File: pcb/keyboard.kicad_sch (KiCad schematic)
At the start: 130 parts, among them J1 Conn_01x04_Pin, J2 AudioJack4, J3 USB_C_Receptacle_USB2.0_16P, J4 AudioJack4, J5 USB_C_Receptacle_USB2.0_16P, J6 Conn_01x04_Pin, SW1 SW_Push, SW10 SW_Push_45deg, SW11 SW_Push_45deg, SW12 SW_Push_45deg, SW13 SW_Push_45deg, SW14 SW_Push_45deg, SW15 SW_Push_45deg, SW16 SW_Push_45deg, SW17 SW_Push_45deg, SW18 SW_Push_45deg, SW19 SW_Push_45deg, SW2 RotaryEncoder_Switch, SW20 SW_Push_45deg, SW21 SW_Push_45deg, SW22 SW_Push_45deg, SW23 SW_Push_45deg, SW24 SW_Push_45deg, SW26 SW_Push_45deg, SW27 SW_Push_45deg, SW28 SW_Push_45deg, SW29 SW_Push_45deg, SW3 SW_Push_45deg, SW30 SW_Push_45deg, SW31 SW_Push_45deg, SW32 SW_Push_45deg, SW33 SW_Push_45deg, SW34 SW_Push_45deg, SW35 SW_Push_45deg, SW36 SW_Push_45deg, SW37 SW_Push_45deg, SW38 RotaryEncoder_Switch, SW39 SW_Push_45deg, SW4 SW_Push_45deg, SW40 SW_Push_45deg, SW41 SW_Push_45deg, SW42 SW_Push_45deg, SW43 SW_Push_45deg, SW44 SW_Push_45deg, SW45 SW_Push_45deg, SW46 SW_Push_45deg, SW47 SW_Push_45deg, SW48 SW_Push_45deg, SW49 SW_Push_45deg, SW5 SW_Push_45deg, SW50 SW_Push_45deg, SW51 SW_Push, SW6 SW_Push_45deg, SW7 SW_Push_45deg, SW8 SW_Push_45deg, SW9 SW_Push_45deg, U2 AMS1117-3.3, U4 STM32F072CBTx, U5 STM32F072CBTx, U6 AMS1117-3.3

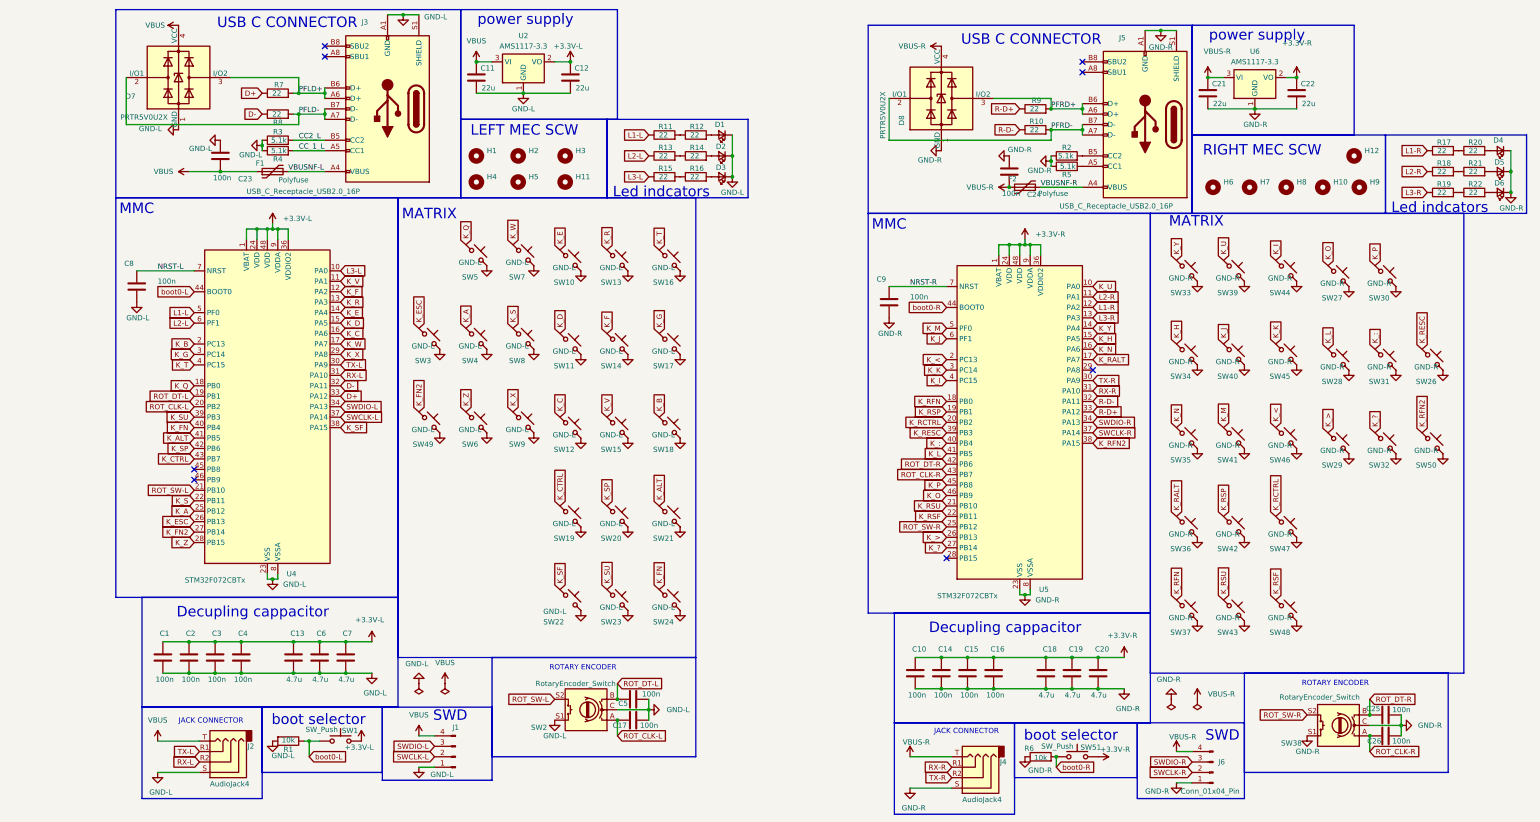
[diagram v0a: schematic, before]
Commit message: init work on rev 3
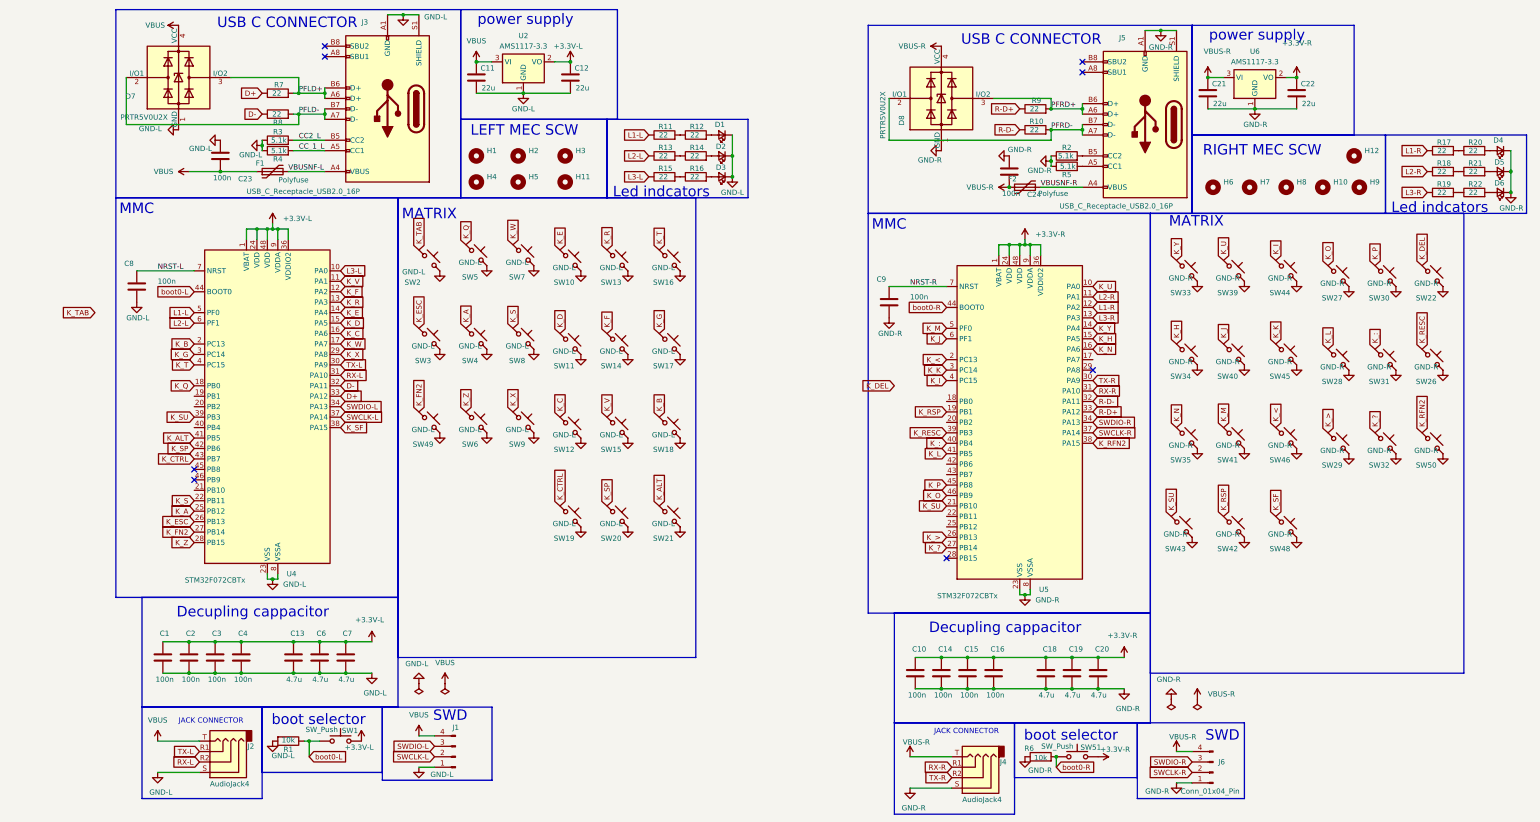
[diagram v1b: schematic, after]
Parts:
- removed C17, C25, C26, C5: 100n, Capacitor_SMD:C_0603_1608Metric, symbol Device:C
- removed SW2, SW38: RotaryEncoder_Switch, PCM_marbastlib-various:ROT_Alps_EC11E-Switch, symbol Device:RotaryEncoder_Switch
- removed SW23, SW24, SW36, SW37, SW47: SW_Push_45deg, PCM_marbastlib-choc:SW_choc_v1_HS_CPG135001S30_1u, symbol Switch:SW_Push_45deg
- added SW2: SW_Push_45deg, PCM_marbastlib-choc:SW_choc_v1_HS_CPG135001S30_1u, symbol Switch:SW_Push_45deg
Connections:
- net K_RSU is gone; now on net K_SU: SW43.1, U5.21 (PB10)
- net GND-L: now also SW2.2; no longer SW22.2
- net GND-R: now also SW22.2
- net K_SF: now also SW48.1; no longer SW22.1
- net K_FN: no longer names the net of U4.40 (PB4)
- net K_RALT: no longer names the net of U5.17 (PA7)
- net K_RCTRL: no longer names the net of U5.20 (PB2)
- net K_RFN: no longer names the net of U5.18 (PB0)
- net K_RSF: no longer names the net of U5.22 (PB11)
- net K_RSF: no longer SW48.1
- net ROT_CLK-L: no longer names the net of U4.20 (PB2)
- net ROT_CLK-R: no longer names the net of U5.43 (PB7)
- net ROT_DT-L: no longer names the net of U4.19 (PB1)
- net ROT_DT-R: no longer names the net of U5.42 (PB6)
- net ROT_SW-L: no longer names the net of U4.21 (PB10)
- net ROT_SW-R: no longer names the net of U5.25 (PB12)
- new net K_DEL: SW22.1
- new net K_TAB: SW2.1
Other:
- note removed: "ROTARY ENCODER"
- moved on the sheet: SW43, SW48

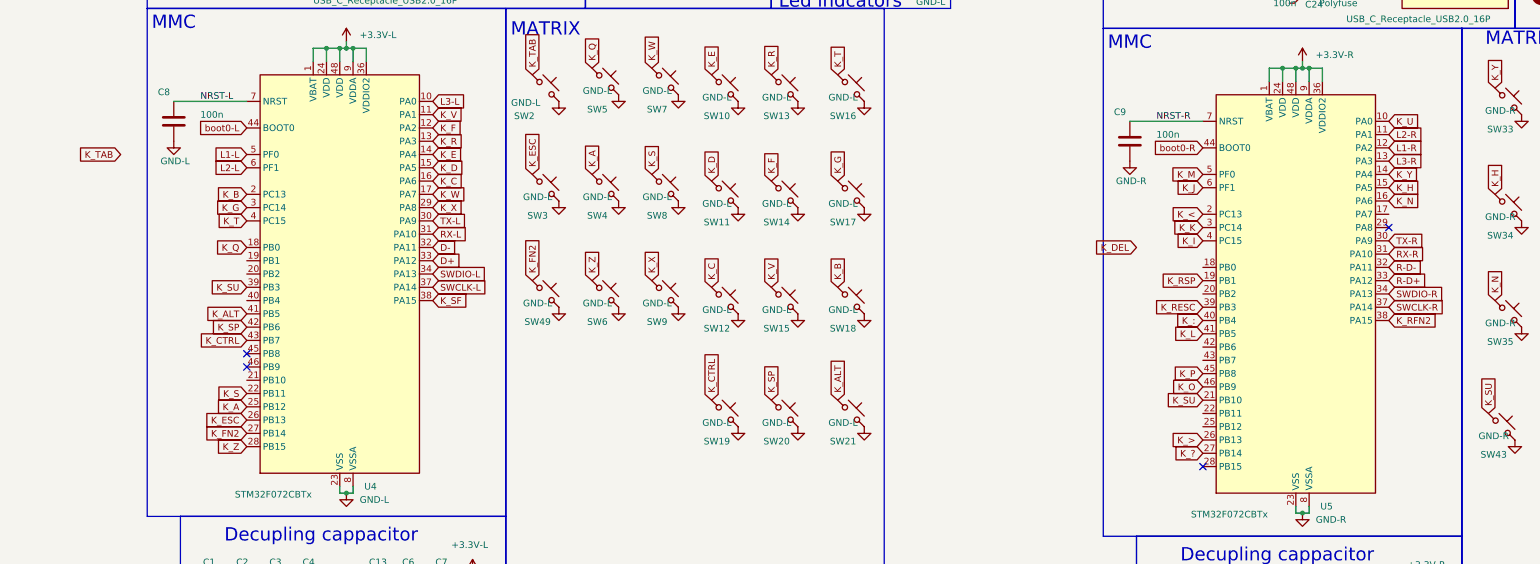
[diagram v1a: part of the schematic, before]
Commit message: pogresss
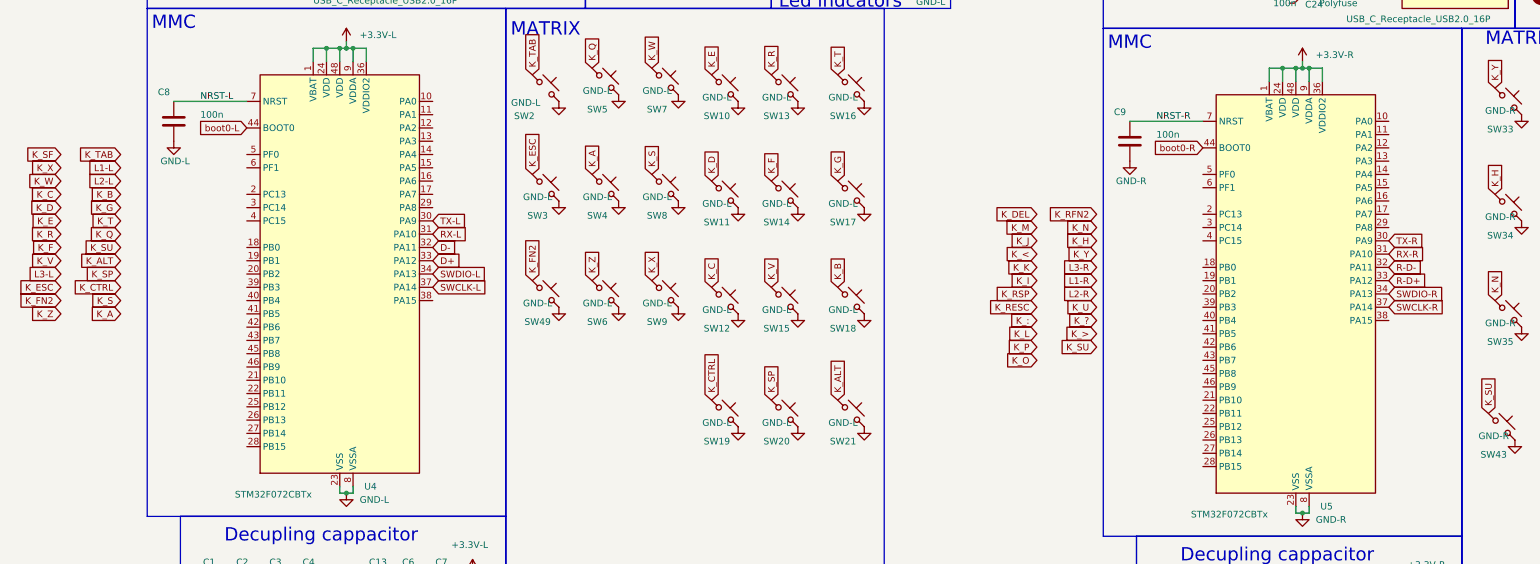
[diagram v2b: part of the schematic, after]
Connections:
- net K_:: no longer U5.40 (PB4)
- net K_<: no longer U5.2 (PC13)
- net K_>: no longer U5.26 (PB13)
- net K_?: no longer U5.27 (PB14)
- net K_A: no longer U4.25 (PB12)
- net K_ALT: no longer U4.41 (PB5)
- net K_B: no longer U4.2 (PC13)
- net K_C: no longer U4.16 (PA6)
- net K_CTRL: no longer U4.43 (PB7)
- net K_D: no longer U4.15 (PA5)
- net K_E : no longer U4.14 (PA4)
- net K_ESC: no longer U4.26 (PB13)
- net K_F: no longer U4.12 (PA2)
- net K_FN2: no longer U4.27 (PB14)
- net K_G: no longer U4.3 (PC14)
- net K_H: no longer U5.15 (PA5)
- net K_I: no longer U5.4 (PC15)
- net K_J: no longer U5.6 (PF1)
- net K_K: no longer U5.3 (PC14)
- net K_L: no longer U5.41 (PB5)
- net K_M: no longer U5.5 (PF0)
- net K_N: no longer U5.16 (PA6)
- net K_O: no longer U5.46 (PB9)
- net K_P: no longer U5.45 (PB8)
- net K_Q: no longer U4.18 (PB0)
- net K_R: no longer U4.13 (PA3)
- net K_RESC: no longer U5.39 (PB3)
- net K_RFN2: no longer U5.38 (PA15)
- net K_RSP: no longer U5.19 (PB1)
- net K_S: no longer U4.22 (PB11)
- net K_SF: no longer U4.38 (PA15)
- net K_SP: no longer U4.42 (PB6)
- net K_SU: no longer U4.39 (PB3), U5.21 (PB10)
- net K_T: no longer U4.4 (PC15)
- net K_U: no longer U5.10 (PA0)
- net K_V: no longer U4.11 (PA1)
- net K_W: no longer U4.17 (PA7)
- net K_X: no longer U4.29 (PA8)
- net K_Y: no longer U5.14 (PA4)
- net K_Z: no longer U4.28 (PB15)
- net L1-L: no longer U4.5 (PF0)
- net L1-R: no longer U5.12 (PA2)
- net L2-L: no longer U4.6 (PF1)
- net L2-R: no longer U5.11 (PA1)
- net L3-L: no longer U4.10 (PA0)
- net L3-R: no longer U5.13 (PA3)
- no-connect marks 8 -> 4
